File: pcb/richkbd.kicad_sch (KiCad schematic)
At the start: 49 parts, among them J1 USB_C_Receptacle, J2 OLED, K0 key-diode-led, K1 key-diode-led, K10 key-diode-led, K11 key-diode-led, K12 key-diode-led, K13 key-diode-led, K14 key-diode-led, K15 key-diode-led, K2 key-diode-led, K20 key-diode-led, K21 key-diode-led, K22 key-diode-led, K23 key-diode-led, K24 key-diode-led, K25 key-diode-led, K3 key-diode-led, K30 key-diode-led, K31 key-diode-led, K32 key-diode-led, K33 key-diode-led, K34 key-diode-led, K35 key-diode-led, K4 key-diode-led, K40 key-diode-led, K41 key-diode-led, K42 key-diode-led, K43 key-diode-led, K44 key-diode-led, K45 key-diode-led, K5 key-diode-led, K50 key-diode-led, K51 key-diode-led, K52 key-diode-led, K53 key-diode-led, K54 key-diode-led, K55 key-diode-led, K60 key-diode-led, K61 key-diode-led, K62 key-diode-led, K63 key-diode-led, K64 key-diode-led, K65 key-diode-led, U1 ProMicro, U2 RP2040_Stamp

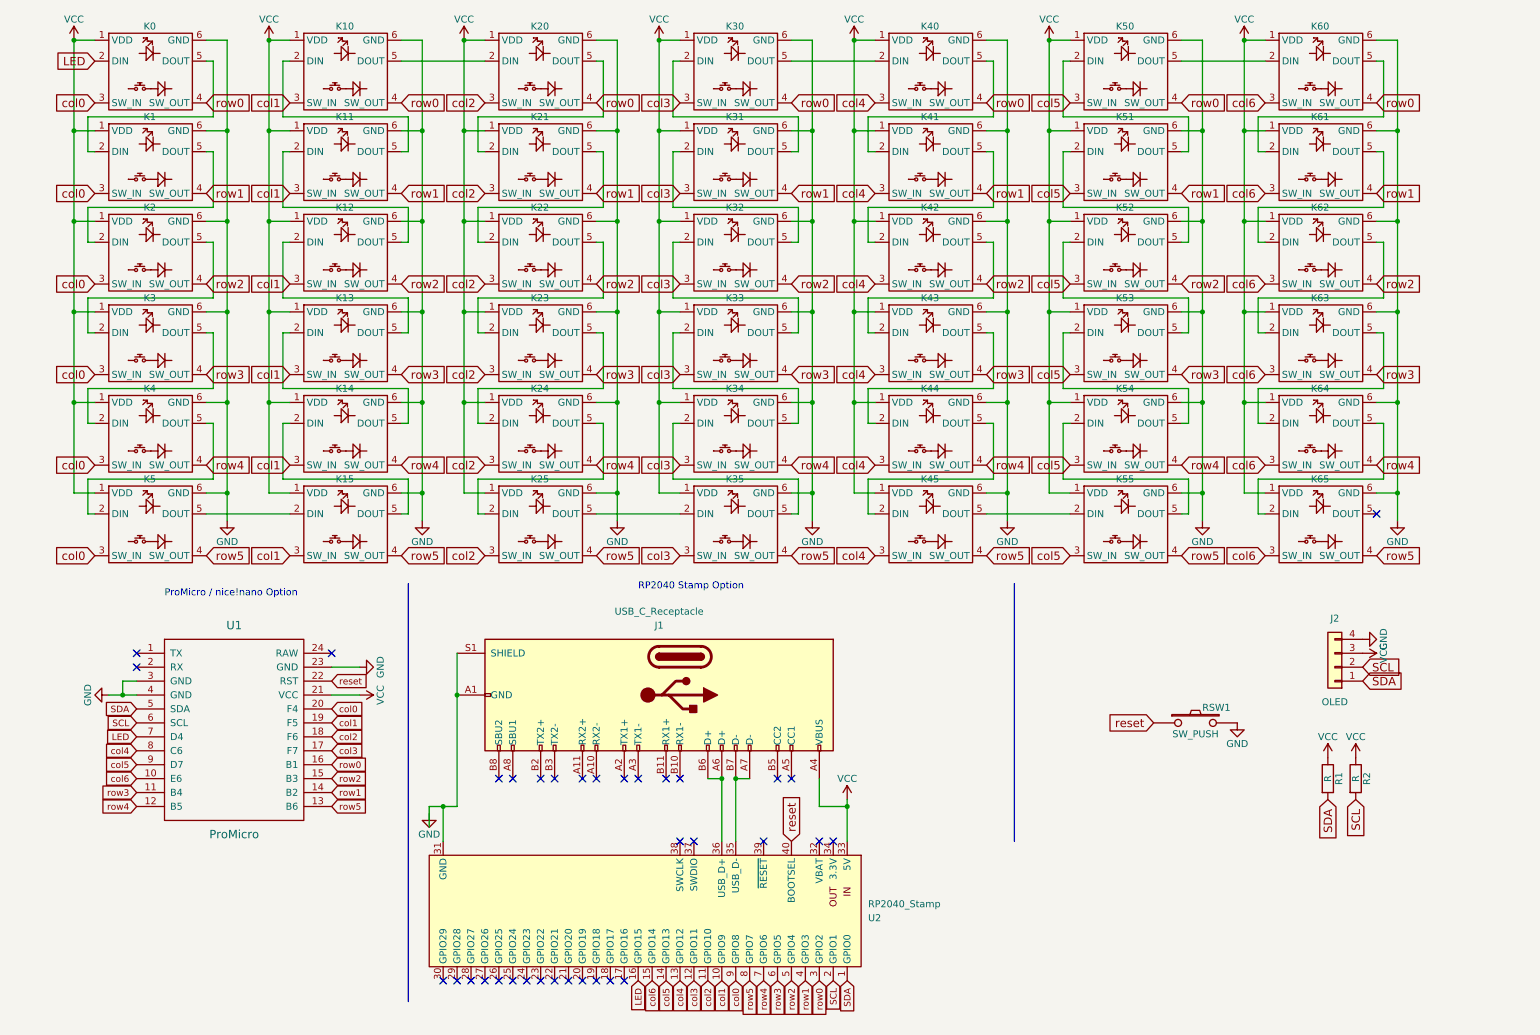
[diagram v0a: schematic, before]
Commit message: Left side routed
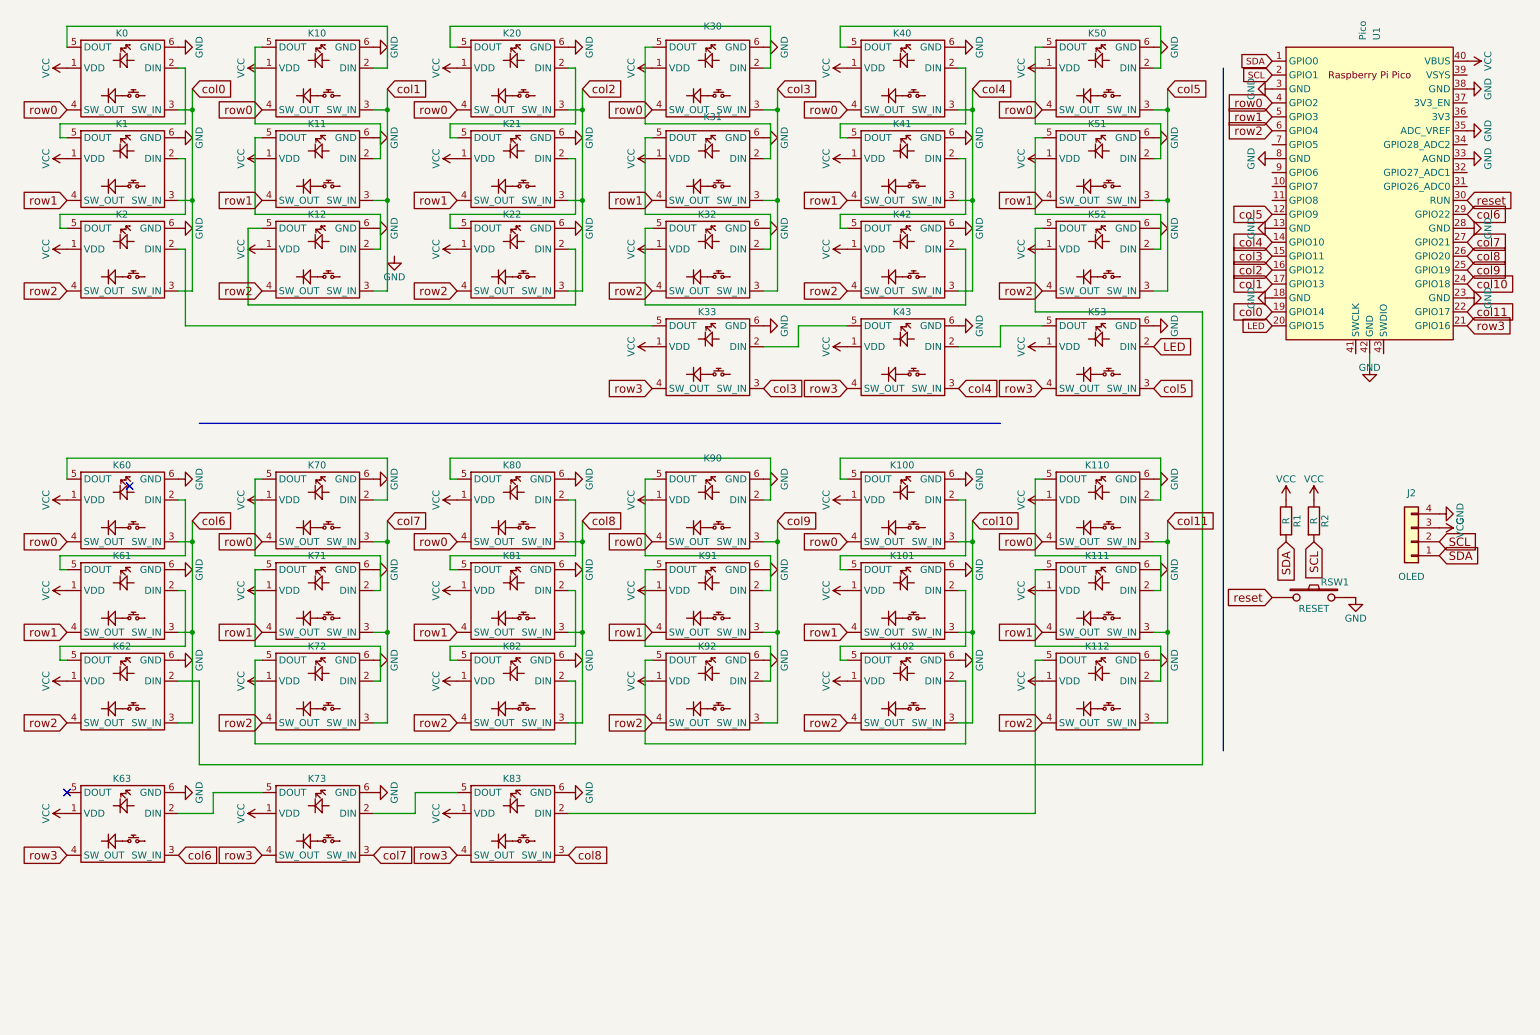
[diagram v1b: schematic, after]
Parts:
- removed J1: USB_C_Receptacle, Connector_USB:USB_C_Receptacle_Amphenol_12401548E4-2A_CircularHoles, symbol Connector:USB_C_Receptacle
- removed K33, K34, K35, K40, K41, K42, K43, K44, K45, K50, K51, K52, K53, K54, K55, K64, K65: key-diode-led, nashlib:key_diode_led, symbol nashlib:key-diode-led
- removed U1: ProMicro, kbd:ProMicro_v2, symbol corne-chocolate-rescue:ProMicro-kbd
- removed U2: RP2040_Stamp, RP2040_Stamp:RP2040_Stamp_SMD, symbol RP2040_Stamp:RP2040_Stamp
- added K100, K101, K102, K110, K111, K112, K70, K71, K72, K73, K80, K81, K82, K83, K90, K91, K92: key-diode-led, nashlib:key_diode_led, symbol nashlib:key-diode-led
- added U1: Pico, MCU_RaspberryPi_and_Boards:RPi_Pico_SMD_TH, symbol MCU_RaspberryPi_and_Boards:Pico
- RSW1: value SW_PUSH -> RESET
- renumbered K3 to K10, K4 to K11, K5 to K12, K10 to K20, K11 to K21, K12 to K22, K13 to K30, K14 to K31, K15 to K32, K32 to K33, K20 to K40, K21 to K41, K22 to K42, K31 to K43, K23 to K50, K24 to K51, K25 to K52, K30 to K53
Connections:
- net row4 is gone; now on net row1: K11.4 (SW_OUT), K31.4 (SW_OUT), K51.4 (SW_OUT)
- net row5 is gone; now on net row2: K12.4 (SW_OUT), K32.4 (SW_OUT), K52.4 (SW_OUT)
- net GND: now also K100.6 (GND), K101.6 (GND), K102.6 (GND), K110.6 (GND), K111.6 (GND), K112.6 (GND), K70.6 (GND), K71.6 (GND), K72.6 (GND), K73.6 (GND), K80.6 (GND), K81.6 (GND), K82.6 (GND), K83.6 (GND), K90.6 (GND), K91.6 (GND), K92.6 (GND), U1.13 (GND), U1.18 (GND), U1.23 (GND), U1.28 (GND), U1.3 (GND), U1.33 (AGND), U1.35 (ADC_VREF), U1.38 (GND), U1.42 (GND), U1.8 (GND)
- net LED: now also K53.2 (DIN), U1.20 (GPIO15); no longer K0.2 (DIN)
- net SCL: now also U1.2 (GPIO1)
- net SDA: now also U1.1 (GPIO0)
- net VCC: now also K100.1 (VDD), K101.1 (VDD), K102.1 (VDD), K110.1 (VDD), K111.1 (VDD), K112.1 (VDD), K70.1 (VDD), K71.1 (VDD), K72.1 (VDD), K73.1 (VDD), K80.1 (VDD), K81.1 (VDD), K82.1 (VDD), K83.1 (VDD), K90.1 (VDD), K91.1 (VDD), K92.1 (VDD), U1.40 (VBUS)
- net col0: now also U1.19 (GPIO14); no longer K10.3 (SW_IN), K11.3 (SW_IN), K12.3 (SW_IN)
- net col1: now also K10.3 (SW_IN), K11.3 (SW_IN), K12.3 (SW_IN), U1.17 (GPIO13); no longer K20.3 (SW_IN), K21.3 (SW_IN), K22.3 (SW_IN), K30.3 (SW_IN), K31.3 (SW_IN), K32.3 (SW_IN)
- net col2: now also K20.3 (SW_IN), K21.3 (SW_IN), K22.3 (SW_IN), U1.16 (GPIO12); no longer K40.3 (SW_IN), K41.3 (SW_IN), K42.3 (SW_IN), K50.3 (SW_IN), K51.3 (SW_IN), K52.3 (SW_IN)
- net col3: now also K30.3 (SW_IN), K31.3 (SW_IN), K32.3 (SW_IN), U1.15 (GPIO11); no longer K43.3 (SW_IN), K53.3 (SW_IN)
- net col4: now also K40.3 (SW_IN), K41.3 (SW_IN), K42.3 (SW_IN), K43.3 (SW_IN), U1.14 (GPIO10)
- net col5: now also K50.3 (SW_IN), K51.3 (SW_IN), K52.3 (SW_IN), K53.3 (SW_IN), U1.12 (GPIO9)
- net col6: now also U1.29 (GPIO22)
- net reset: now also U1.30 (RUN)
- net row0: now also K10.4 (SW_OUT), K30.4 (SW_OUT), K50.4 (SW_OUT), K100.4 (SW_OUT), K110.4 (SW_OUT), K70.4 (SW_OUT), K80.4 (SW_OUT), K90.4 (SW_OUT), U1.4 (GPIO2); no longer K53.4 (SW_OUT)
- net row1: now also K101.4 (SW_OUT), K111.4 (SW_OUT), K71.4 (SW_OUT), K81.4 (SW_OUT), K91.4 (SW_OUT), U1.5 (GPIO3); no longer K43.4 (SW_OUT)
- net row2: now also K102.4 (SW_OUT), K112.4 (SW_OUT), K72.4 (SW_OUT), K82.4 (SW_OUT), K92.4 (SW_OUT), U1.6 (GPIO4); no longer K33.4 (SW_OUT)
- net row3: now also K33.4 (SW_OUT), K43.4 (SW_OUT), K53.4 (SW_OUT), K73.4 (SW_OUT), K83.4 (SW_OUT), U1.21 (GPIO16); no longer K10.4 (SW_OUT), K30.4 (SW_OUT), K50.4 (SW_OUT)
- net at K61.5 (DOUT): now also K60.2 (DIN); no longer K62.2 (DIN)
- net at K62.5 (DOUT): now also K61.2 (DIN); no longer K63.2 (DIN)
- net at K2.2 (DIN): now also K33.5 (DOUT); no longer K1.5 (DOUT)
- net at K2.5 (DOUT): now also K1.2 (DIN); no longer K10.2 (DIN)
- net at K43.2 (DIN): now also K53.5 (DOUT); no longer K33.5 (DOUT)
- net at K43.5 (DOUT): now also K33.2 (DIN); no longer K53.2 (DIN)
- net at K50.2 (DIN): now also K40.5 (DOUT); no longer K42.5 (DOUT)
- net at K52.5 (DOUT): now also K62.2 (DIN)
- net at K0.5 (DOUT): now also K10.2 (DIN); no longer K1.2 (DIN)
- net at K22.2 (DIN): now also K12.5 (DOUT); no longer K30.5 (DOUT)
- net at K40.2 (DIN): now also K41.5 (DOUT); no longer K20.5 (DOUT)
- net at K41.2 (DIN): now also K42.5 (DOUT); no longer K40.5 (DOUT)
- net at K32.2 (DIN): now also K31.5 (DOUT); no longer K12.5 (DOUT)
- net at K60.5 (DOUT): now also K70.2 (DIN); no longer K61.2 (DIN)
- net at K42.2 (DIN): now also K32.5 (DOUT); no longer K41.5 (DOUT)
- net at K31.2 (DIN): now also K30.5 (DOUT); no longer K32.5 (DOUT)
- net at K30.2 (DIN): now also K20.5 (DOUT); no longer K31.5 (DOUT)
- new net: K100.2 (DIN), K101.5 (DOUT)
- new net: K100.5 (DOUT), K110.2 (DIN)
- new net: K80.2 (DIN), K81.5 (DOUT)
- new net: K80.5 (DOUT), K90.2 (DIN)
- new net: K63.2 (DIN), K73.5 (DOUT)
- new net: K73.2 (DIN), K83.5 (DOUT)
- new net: K110.5 (DOUT), K111.2 (DIN)
- new net: K71.5 (DOUT), K72.2 (DIN)
- new net: K72.5 (DOUT), K82.2 (DIN)
- new net: K81.2 (DIN), K82.5 (DOUT)
- new net: K112.5 (DOUT), K83.2 (DIN)
- new net: K0.2 (DIN), K1.5 (DOUT)
- new net: K90.5 (DOUT), K91.2 (DIN)
- new net: K91.5 (DOUT), K92.2 (DIN)
- new net: K102.2 (DIN), K92.5 (DOUT)
- new net: K101.2 (DIN), K102.5 (DOUT)
- new net: K70.5 (DOUT), K71.2 (DIN)
- new net: K111.5 (DOUT), K112.2 (DIN)
- new net col10: K100.3 (SW_IN), K101.3 (SW_IN), K102.3 (SW_IN), U1.24 (GPIO18)
- new net col11: K110.3 (SW_IN), K111.3 (SW_IN), K112.3 (SW_IN), U1.22 (GPIO17)
- new net col7: K70.3 (SW_IN), K71.3 (SW_IN), K72.3 (SW_IN), K73.3 (SW_IN), U1.27 (GPIO21)
- new net col8: K80.3 (SW_IN), K81.3 (SW_IN), K82.3 (SW_IN), K83.3 (SW_IN), U1.26 (GPIO20)
- new net col9: K90.3 (SW_IN), K91.3 (SW_IN), K92.3 (SW_IN), U1.25 (GPIO19)
- no-connect marks 35 -> 2
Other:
- note removed: "ProMicro / nice!nano Option"
- note removed: "RP2040 Stamp Option"
- moved on the sheet: J2, K0, K10, K11, K12, K2, K20, K21, K22, K30, K31, K32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
